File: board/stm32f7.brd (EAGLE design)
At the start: 49.7 x 49.8 mm, 38 parts, among them IC1 LM2937, IC2 FT232RL, U1 STM32F722XX, X1 MINI-USB-32005-201, X2 MINI-USB-32005-201

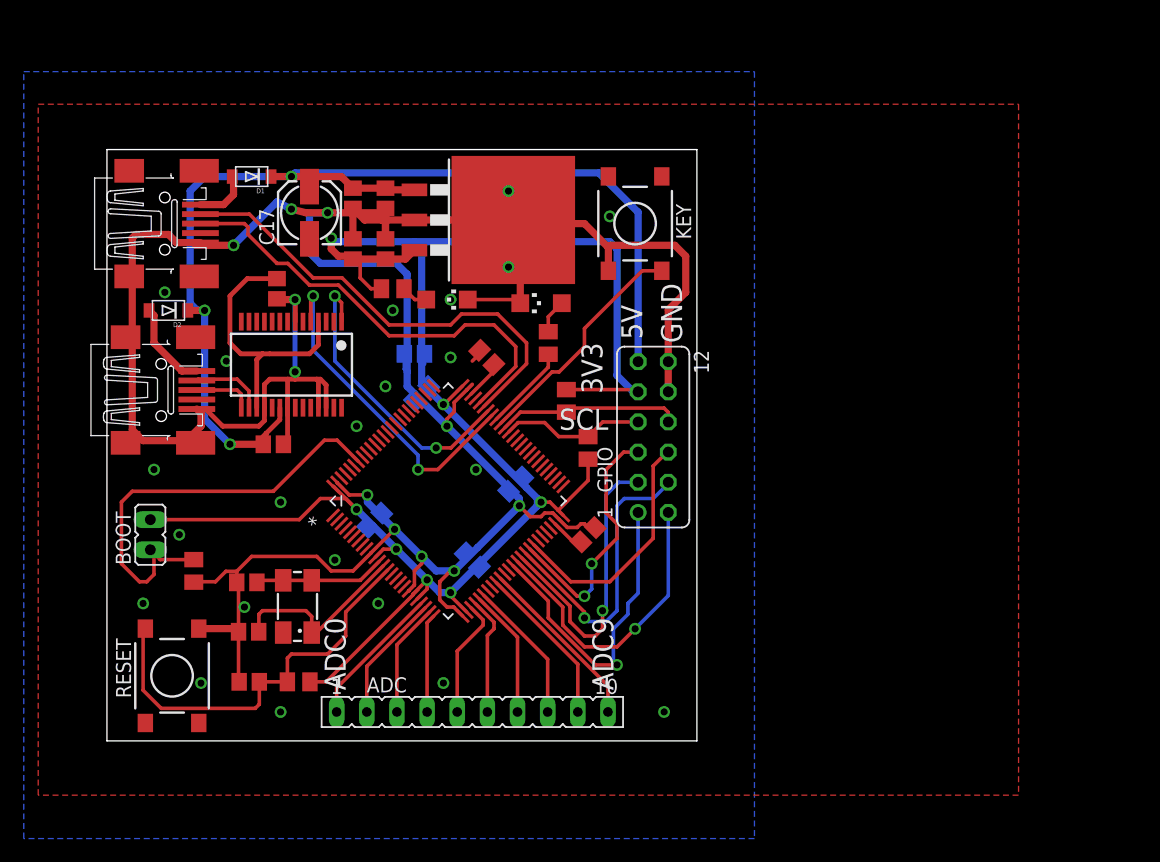
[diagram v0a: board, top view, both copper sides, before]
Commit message: common
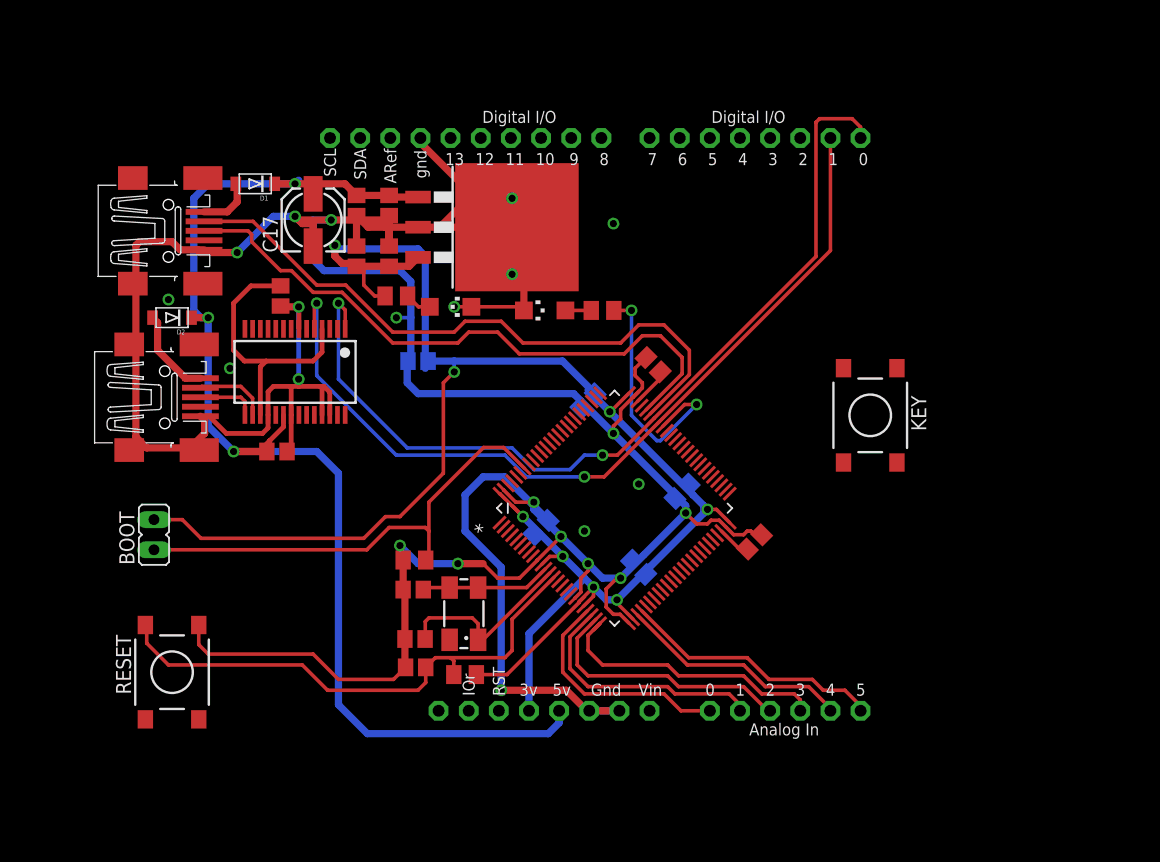
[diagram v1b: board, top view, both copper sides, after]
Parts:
- removed ADC: (no value), con-lsta:FE10
- removed GPIO: (no value), con-lsta:FE06-2
- removed R4, R5: 4k7, resistor:M0805
- added U2: ARDUINOR3-BPLACE, adafruit:ARDUINOR3-BPLACE
- moved KEY 25.6 mm to (64.3, 27.4)
- moved R2 18.6 mm to (25.9, 15.2), turned to 0 degrees
- moved C3 14.1 mm to (26.0, 6.20)
- moved C5 14.0 mm to (46.0, 31.7)
- moved C7 14.0 mm to (48.5, 21.0)
- moved C8 14.0 mm to (40.5, 28.7)
- moved C9 14.0 mm to (36.6, 18.0)
- moved R1 14.0 mm to (30.2, 5.59)
- moved U1 14.0 mm to (42.8, 19.6)
- moved C1 14.0 mm to (26.0, 8.59)
- moved C2 14.0 mm to (25.8, 12.8)
- moved C6 14.0 mm to (44.8, 14.6)
- moved Q1 14.0 mm to (30.1, 10.7)
- moved C4 14.0 mm to (54.6, 16.8)
- moved R3 5.33 mm to (41.8, 36.3), turned to 0 degrees
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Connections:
- new net N$14: U2.D2
- new net N$15: U2.D3
- new net N$16: U2.D4
- new net N$17: U2.D5
- new net N$18: U2.D6
- new net N$19: U2.D7
- new net N$20: U2.D8
- new net N$21: U2.D9
- new net N$22: U2.D10
- new net N$23: U2.D11
- new net N$24: U2.D12
- new net N$25: U2.D13
- new net VIN: U2.VIN
- net +3V3: now also U2.3V; no longer GPIO.9, R4.2, R5.2
- net +5V: now also U2.5V; no longer GPIO.11
- net ADC0: now also U2.A0; no longer ADC.1
- net ADC1: now also U2.A1; no longer ADC.2
- net ADC2: now also U2.A2; no longer ADC.3
- net ADC3: now also U2.A3; no longer ADC.4
- net ADC4: now also U2.A4; no longer ADC.5
- net ADC5: now also U2.A5; no longer ADC.6
- net ADC6: no longer ADC.7
- net ADC7: no longer ADC.8
- net ADC8: no longer ADC.9
- net ADC9: no longer ADC.10
- net GND: now also U2.GND, U2.GND1, U2.GND2; no longer GPIO.10, GPIO.12
- net SCL: no longer GPIO.7, R5.1
- net SDA: no longer GPIO.8, R4.1
- net TIM1_CH1: no longer GPIO.2
- net TIM1_CH1N: no longer GPIO.1
- net TIM1_CH2: no longer GPIO.4
- net TIM1_CH2N: no longer GPIO.3
- net TIM1_CH3: no longer GPIO.6
- net TIM1_CH3N: no longer GPIO.5
- net USART1_RX: now also U2.D0
- net USART1_TX: now also U2.D1
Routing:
- net GND: track 267.0 -> 321.9 mm, vias 33 -> 23
- net USART1_RX: track 25.1 -> 76.0 mm
- net USART1_TX: track 28.7 -> 72.5 mm
- net TIM1_CH1N: track 26.9 -> 0.00 mm, vias 1 -> 0
- net TIM1_CH1: track 25.4 -> 0.00 mm, vias 1 -> 0
- net TIM1_CH2N: track 25.1 -> 0.00 mm, vias 1 -> 0
- net TIM1_CH2: track 24.8 -> 0.00 mm, vias 1 -> 0
- net TIM1_CH3N: track 21.7 -> 0.00 mm, vias 2 -> 0
- net TIM1_CH3: track 20.7 -> 0.00 mm
- net KEY: track 19.8 -> 0.00 mm
- net ADC3: track 8.31 -> 24.0 mm
- net SDA: track 15.4 -> 0.00 mm
- net ADC9: track 15.0 -> 0.00 mm
- net USBDP: track 38.0 -> 52.8 mm
- net USBDM: track 39.6 -> 54.2 mm
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- removed copper zone on layer 1, net GND
- removed copper zone on layer 16, net GND
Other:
- board outline removed
- board text removed: "3V3"
- board text removed: "5V"
- board text removed: "ADC0"
- board text removed: "ADC9"
- board text removed: "GND"
- board text removed: "SCL"

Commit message: board
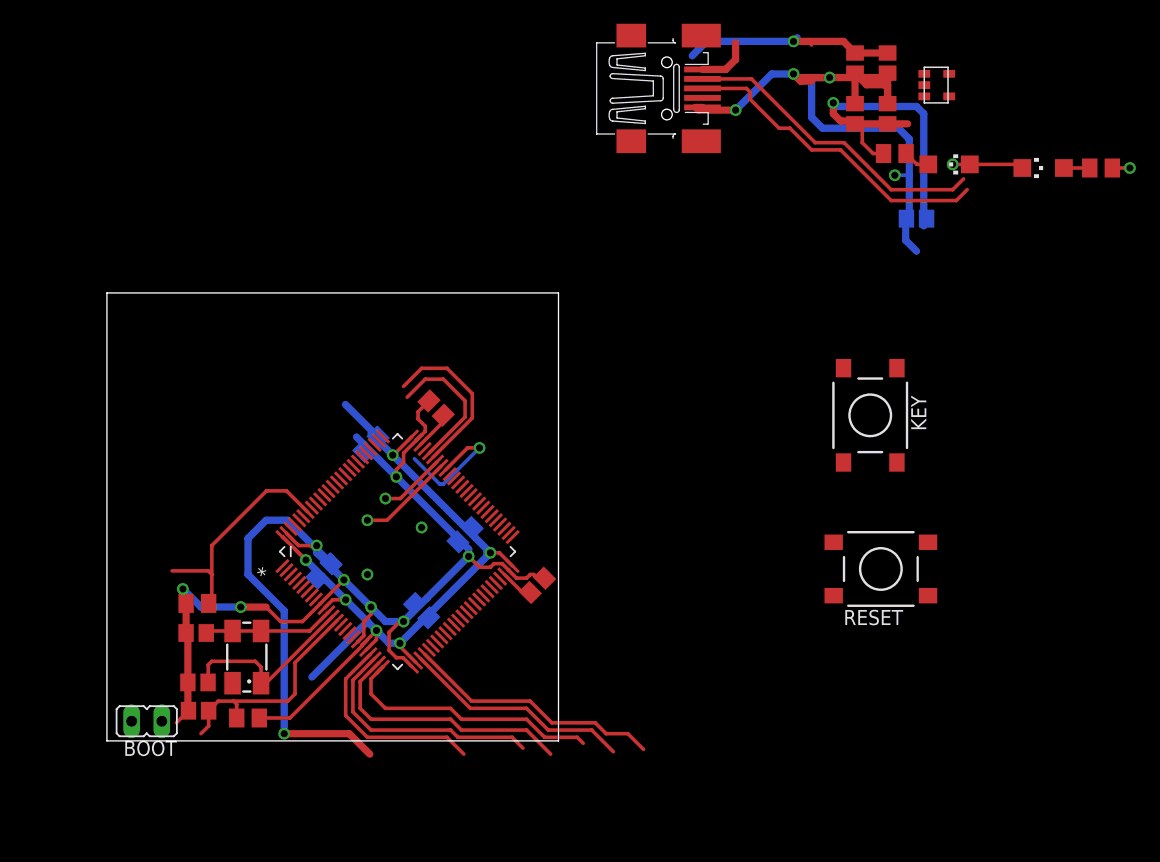
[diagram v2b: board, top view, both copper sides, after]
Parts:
- removed C14: 100n, resistor:C0805
- removed C15: 10uF, resistor:C0805
- removed C17: 22uF, resistor:153CLV-0505
- removed D1, D2: (no value), adafruit:SOD-123FL
- removed IC1: LM2937, linear:TO263-3
- removed IC2: FT232RL, ftdichip:SSOP28
- removed U2: ARDUINOR3-BPLACE, adafruit:ARDUINOR3-BPLACE
- removed X2: MINI-USB-32005-201, con-cypressindustries:32005-201
- added U$1: MIC5504-3.3Y, my_parts:SOT23-5
- moved RESET 60.4 mm to (65.2, 14.5), turned to 0 degrees
- moved C10 43.7 mm to (65.8, 57.1)
- moved C11 43.7 mm to (63.0, 57.1)
- moved C12 43.7 mm to (65.8, 52.8)
- moved C13 43.7 mm to (63.0, 52.8)
- moved C16 43.7 mm to (68.2, 44.0)
- moved LED2 43.7 mm to (71.0, 48.6)
- moved R3 43.7 mm to (83.8, 48.3)
- moved R6 43.7 mm to (66.4, 49.5)
- moved X1 43.7 mm to (47.2, 55.0)
- moved LED1 43.7 mm to (78.9, 48.3)
- moved C8 18.7 mm to (22.3, 25.0)
- moved C1 18.7 mm to (7.67, 4.93)
- moved C2 18.7 mm to (7.52, 9.09)
- moved C3 18.7 mm to (7.72, 2.54)
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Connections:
- removed net N$10: D2.A, X2.1
- removed net N$14: U2.D2
- removed net N$15: U2.D3
- removed net N$16: U2.D4
- removed net N$17: U2.D5
- removed net N$18: U2.D6
- removed net N$19: U2.D7
- removed net N$20: U2.D8
- removed net N$21: U2.D9
- removed net N$22: U2.D10
- removed net N$23: U2.D11
- removed net N$24: U2.D12
- removed net N$25: U2.D13
- removed net N$6: C14.1, IC2.17, IC2.4
- removed net N$7: D1.A, X1.1
- removed net N$8: IC2.16, X2.2
- removed net N$9: IC2.15, X2.3
- removed net VIN: U2.VIN
- net +3V3: now also U$1.P$5; no longer IC1.3, U2.3V
- net +5V: now also U$1.P$1, U$1.P$3, X1.1; no longer C15.1, C17.+, D1.C, D2.C, IC1.1, IC2.20, U2.5V
- net ADC0: no longer U2.A0
- net ADC1: no longer U2.A1
- net ADC2: no longer U2.A2
- net ADC3: no longer U2.A3
- net ADC4: no longer U2.A4
- net ADC5: no longer U2.A5
- net GND: now also U$1.P$2; no longer C14.2, C15.2, C17.-, IC1.2, IC2.18, IC2.21, IC2.25, IC2.26, IC2.7, U2.GND, U2.GND1, U2.GND2, X2.5
- net USART1_RX: no longer IC2.1, U2.D0
- net USART1_TX: no longer IC2.5, U2.D1
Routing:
- net GND: track 321.9 -> 190.2 mm, vias 23 -> 16
- net +5V: track 104.5 -> 23.0 mm, vias 3 -> 1
- net USART1_RX: track 76.0 -> 5.64 mm, vias 2 -> 1
- net USART1_TX: track 72.5 -> 8.14 mm, vias 2 -> 1
- net +3V3: track 162.3 -> 106.3 mm, vias 8 -> 7
- net RESET: track 45.3 -> 19.2 mm
- net N$6: track 23.4 -> 0.00 mm
- net BOOT: track 39.8 -> 19.2 mm
- net USBDM: track 54.2 -> 40.3 mm
- net USBDP: track 52.8 -> 38.9 mm
- net LED: track 21.6 -> 12.8 mm
- net N$10: track 7.50 -> 0.00 mm
- net N$8: track 6.27 -> 0.00 mm
- net N$9: track 5.04 -> 0.00 mm
- net N$7: track 4.71 -> 0.00 mm
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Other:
- board outline added: 38 x 37.7 mm
